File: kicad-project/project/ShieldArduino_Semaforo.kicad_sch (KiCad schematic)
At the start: 101 parts, among them IC1 TLIN1039DDFRQ1, IC2 TPS563200DDCR, IC3 MCP4901T-E_MS, J2 Conn_01x18, K1 RELAY, P1 Power, P2 Analog, P3 Digital, P4 Digital, P5 CONN_01X01, P6 CONN_01X01, P7 CONN_01X01, P8 CONN_01X01, Q1 PMOS, Q2 NMOS, Q3 NMOS, Q4 NMOS, Q5 NMOS, U1 MCP2542FD-E/MF, U3 LM4040DBZ-2.0

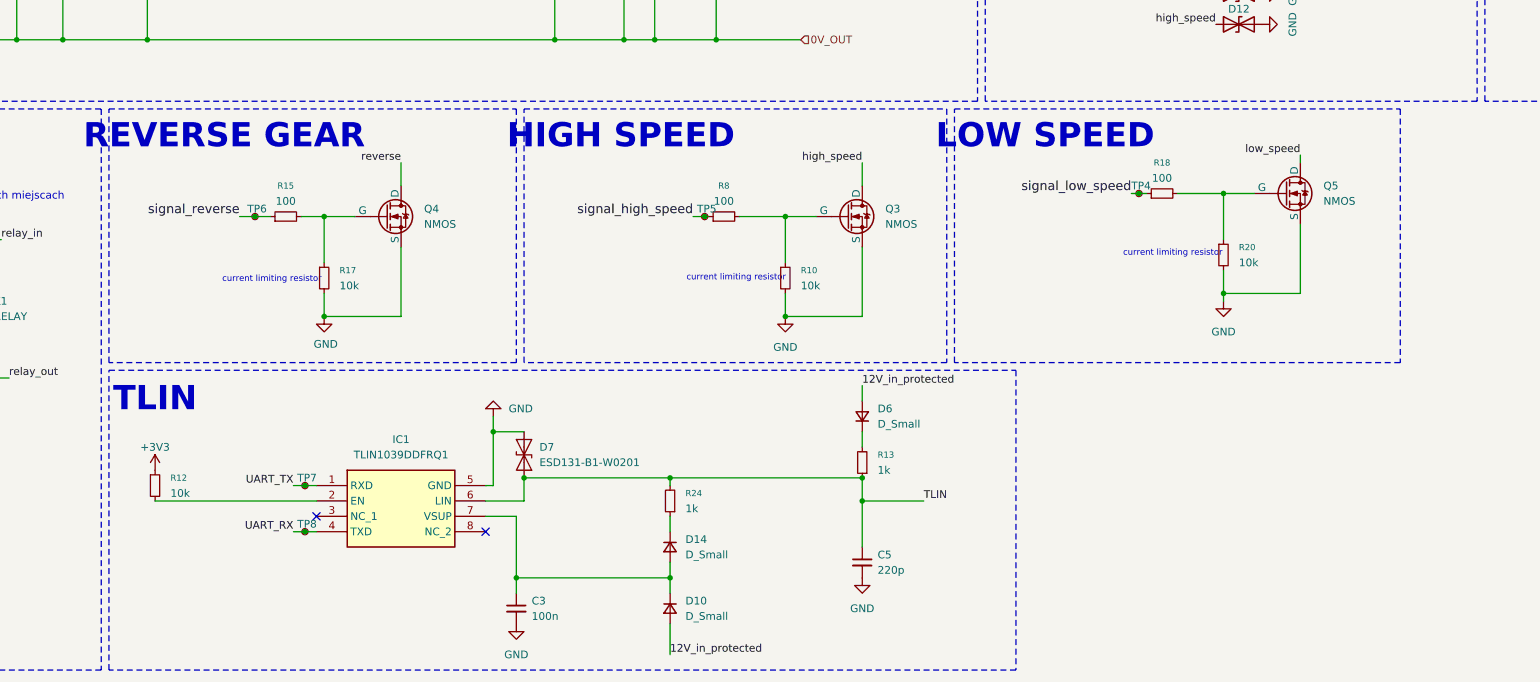
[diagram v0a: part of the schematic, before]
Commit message: kicad-schemat-work
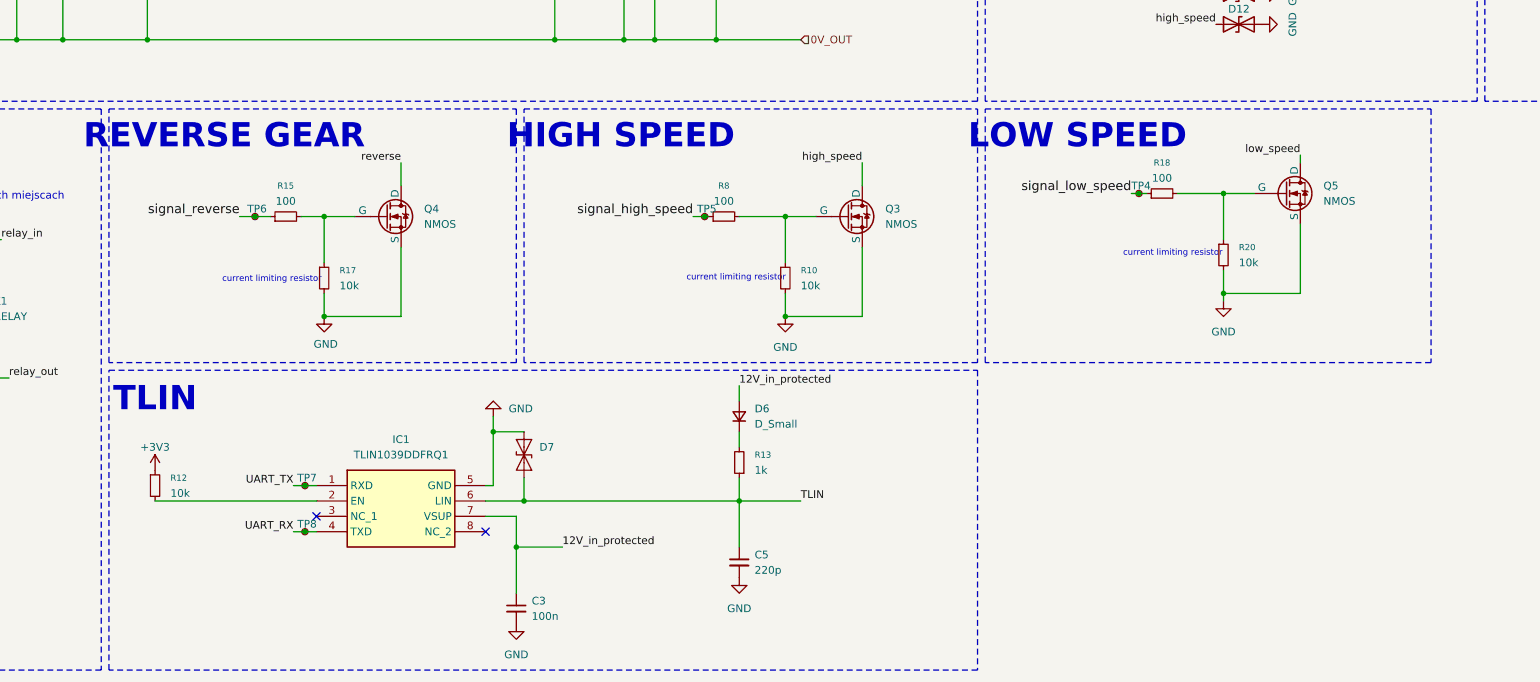
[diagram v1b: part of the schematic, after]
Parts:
- removed D10, D14: D_Small, symbol Device:D_Small
- removed R24: 1k, Resistor_SMD:R_0805_2012Metric_Pad1.20x1.40mm_HandSolder, symbol Device:R_Small
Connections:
- net 12V_in_protected: now also C3.1, IC1.7 (VSUP)
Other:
- moved on the sheet: C5, D6, R13
